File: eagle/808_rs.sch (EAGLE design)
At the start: 75 parts, among them IC1 TL072P, IC2 TL072P, Q1 2SK30, Q59 2N3904, Q60 2N3906, Q61 2N3904, Q62 2N3904, Q63 2N3904, SW8 808_LT_MSS42_SW_4PDT

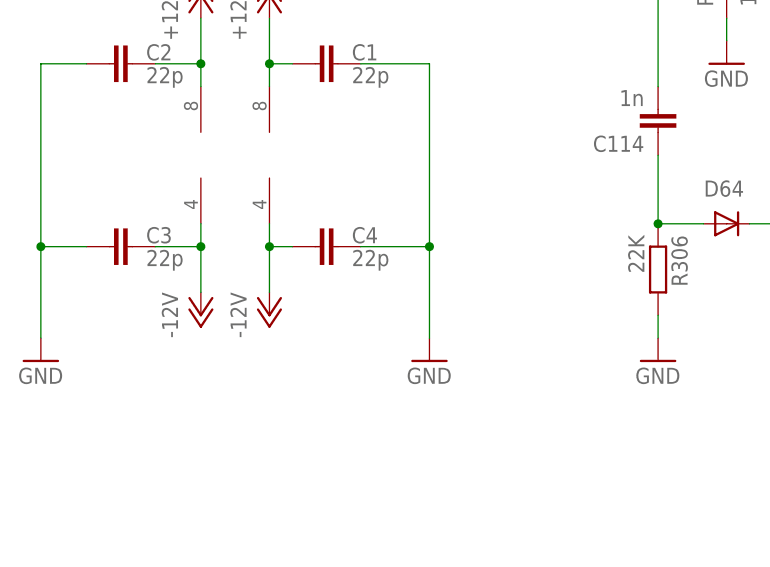
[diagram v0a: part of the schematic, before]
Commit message: 93pct auto
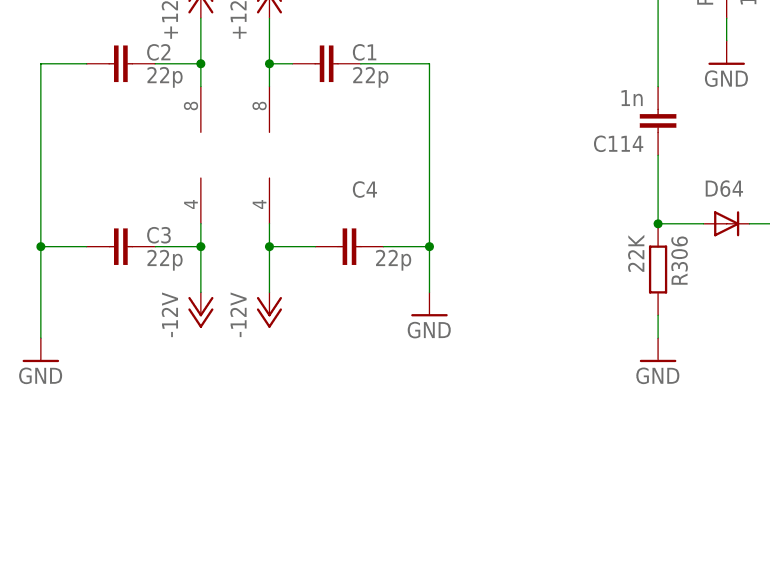
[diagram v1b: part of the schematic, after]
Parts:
- R305, R306, R310, R311, R316, R323, R324, R325, R326, R331: device TR808clone:R-EU_0207/5V -> TR808clone:R-EU_0207/7
- R313: device TR808clone:R-EU_0207/5V -> TR808clone:R-EU_0309/12
- R318: device TR808clone:R-EU_0207/5V -> TR808clone:R-EU_0207/2V
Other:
- moved on the sheet: C4

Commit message: 95pct auto
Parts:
- C113: device TR808clone:C-EU050-024X044 -> TR808clone:C-EU075-032X103
- C114: device TR808clone:C-EU3.5MM_PITCH -> TR808clone:C-EU050-030X075
- C121: device TR808clone:C-EU3.5MM_PITCH -> TR808clone:C-EU050-025X075
- C4: device TR808clone:C-EU025-025X050 -> TR808clone:C-EU050-024X044
- D61, D63, D64: value 1N4148DO35-7 -> 1N4148DO35-10; device TR808clone:1N4148DO35-7 -> TR808clone:1N4148DO35-10
- R303, R309, R330: device TR808clone:R-EU_0207/5V -> TR808clone:R-EU_0207/2V
- R316: device TR808clone:R-EU_0207/7 -> TR808clone:R-EU_0207/5V
- R321: device TR808clone:R-EU_0207/5V -> TR808clone:R-EU_0207/7
- R326: device TR808clone:R-EU_0207/7 -> TR808clone:R-EU_0309/10
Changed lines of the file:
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@@
 <part name="Q59" library="808_lt" deviceset="2N3904" device=""/>
 <part name="Q60" library="808_lt" deviceset="2N3906" device=""/>
-<part name="R303" library="TR808clone" deviceset="R-EU_" device="0207/5V" value="10K"/>
+<part name="R303" library="TR808clone" deviceset="R-EU_" device="0207/2V" value="10K"/>
 <part name="R297" library="TR808clone" deviceset="R-EU_" device="0207/5V" value="22K"/>
 <part name="R299" library="TR808clone" deviceset="R-EU_" device="0207/5V" value="4K7"/>
@@
 <part name="V200" library="supply1" deviceset="GND" device=""/>
 <part name="V201" library="supply1" deviceset="GND" device=""/>
-<part name="D61" library="TR808clone" deviceset="1N4148" device="DO35-7"/>
+<part name="D61" library="TR808clone" deviceset="1N4148" device="DO35-10" value="1N4148DO35-10"/>
 <part name="V202" library="supply1" deviceset="GND" device=""/>
 <part name="R107" library="TR808clone" deviceset="R-EU_" device="0207/5V" value="1K"/>
 <part name="V203" library="supply1" deviceset="GND" device=""/>
 <part name="R108" library="TR808clone" deviceset="R-EU_" device="0207/5V" value="10K"/>
-<part name="D63" library="TR808clone" deviceset="1N4148" device="DO35-7"/>
-<part name="C121" library="TR808clone" deviceset="C-EU" device="3.5MM_PITCH" value="4.7n"/>
+<part name="D63" library="TR808clone" deviceset="1N4148" device="DO35-10" value="1N4148DO35-10"/>
+<part name="C121" library="TR808clone" deviceset="C-EU" device="050-025X075" value="4.7n"/>
 <part name="C122" library="TR808clone" deviceset="C-EU" device="3.5MM_PITCH" value="4.7n"/>
 <part name="R325" library="TR808clone" deviceset="R-EU_" device="0207/7" value="330K"/>
@@
 <part name="V208" library="supply1" deviceset="GND" device=""/>
 <part name="R301" library="TR808clone" deviceset="R-EU_" device="0207/5V" value="47K"/>
-<part name="C114" library="TR808clone" deviceset="C-EU" device="3.5MM_PITCH" value="1n"/>
+<part name="C114" library="TR808clone" deviceset="C-EU" device="050-030X075" value="1n"/>
 <part name="R306" library="TR808clone" deviceset="R-EU_" device="0207/7" value="22K"/>
-<part name="D64" library="TR808clone" deviceset="1N4148" device="DO35-7"/>
+<part name="D64" library="TR808clone" deviceset="1N4148" device="DO35-10" value="1N4148DO35-10"/>
 <part name="R310" library="TR808clone" deviceset="R-EU_" device="0207/7" value="33K"/>
 <part name="R311" library="TR808clone" deviceset="R-EU_" device="0207/7" value="10K"/>
@@
 <part name="R313" library="TR808clone" deviceset="R-EU_" device="0309/12" value="390K"/>
 <part name="V212" library="supply1" deviceset="GND" device=""/>
-<part name="R309" library="TR808clone" deviceset="R-EU_" device="0207/5V" value="33K"/>
+<part name="R309" library="TR808clone" deviceset="R-EU_" device="0207/2V" value="33K"/>
 <part name="R319" library="TR808clone" deviceset="R-EU_" device="0207/5V" value="220K"/>
 <part name="C125" library="TR808clone" deviceset="C-EU" device="3.5MM_PITCH" value="10n"/>
-<part name="R326" library="TR808clone" deviceset="R-EU_" device="0207/7" value="10K"/>
+<part name="R326" library="TR808clone" deviceset="R-EU_" device="0309/10" value="10K"/>
 <part name="R331" library="TR808clone" deviceset="R-EU_" device="0207/7" value="47K"/>
 <part name="V213" library="supply1" deviceset="GND" device=""/>
 <part name="C153" library="TR808clone" deviceset="C-EU" device="025-025X050" value="22p"/>
-<part name="R330" library="TR808clone" deviceset="R-EU_" device="0207/5V" value="470K"/>
+<part name="R330" library="TR808clone" deviceset="R-EU_" device="0207/2V" value="470K"/>
 <part name="C126" library="TR808clone" deviceset="CPOL-EU" device="E2.5-5" value="33/6.3"/>
 <part name="C116" library="TR808clone" deviceset="C-EU" device="3.5MM_PITCH" value="4.7n"/>
@@
 <part name="R315" library="TR808clone" deviceset="R-EU_" device="0207/5V" value="5K6"/>
 <part name="V214" library="supply1" deviceset="GND" device=""/>
-<part name="R316" library="TR808clone" deviceset="R-EU_" device="0207/7" value="1M"/>
+<part name="R316" library="TR808clone" deviceset="R-EU_" device="0207/5V" value="1M"/>
 <part name="R318" library="TR808clone" deviceset="R-EU_" device="0207/2V" value="220K"/>
 <part name="R317" library="TR808clone" deviceset="R-EU_" device="0207/5V" value="10K"/>
 <part name="Q62" library="808_lt" deviceset="2N3904" device=""/>
 <part name="V215" library="supply1" deviceset="GND" device=""/>
-<part name="R321" library="TR808clone" deviceset="R-EU_" device="0207/5V" value="2M2"/>
+<part name="R321" library="TR808clone" deviceset="R-EU_" device="0207/7" value="2M2"/>
 <part name="C120" library="TR808clone" deviceset="CPOL-EU" device="E2.5-5" value="10/16"/>
 <part name="V217" library="supply1" deviceset="GND" device=""/>
@@
 <part name="Q61" library="808_lt" deviceset="2N3904" device=""/>
 <part name="C112" library="TR808clone" deviceset="C-EU" device="050-024X044" value="22n"/>
-<part name="C113" library="TR808clone" deviceset="C-EU" device="050-024X044" value="47n"/>
+<part name="C113" library="TR808clone" deviceset="C-EU" device="075-032X103" value="47n"/>
 <part name="R304" library="TR808clone" deviceset="R-EU_" device="0207/5V" value="47K"/>
 <part name="R305" library="TR808clone" deviceset="R-EU_" device="0207/7" value="1M"/>
@@
 <part name="C2" library="TR808clone" deviceset="C-EU" device="025-025X050" value="22p"/>
 <part name="C3" library="TR808clone" deviceset="C-EU" device="025-025X050" value="22p"/>
-<part name="C4" library="TR808clone" deviceset="C-EU" device="025-025X050" value="22p"/>
+<part name="C4" library="TR808clone" deviceset="C-EU" device="050-024X044" value="22p"/>
 <part name="TRIGGER" library="solpad" deviceset="LSP11" device=""/>
 <part name="SW8" library="808_lt" deviceset="808_LT_MSS42_SW_4PDT" device=""/>

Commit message: 94pct auto
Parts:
- C118: device TR808clone:C-EU3.5MM_PITCH -> TR808clone:C-EU050-024X044
- C122: device TR808clone:C-EU3.5MM_PITCH -> TR808clone:C-EU050-030X075
- R318: device TR808clone:R-EU_0207/2V -> TR808clone:R-EU_0207/5V
- R320, R322: device TR808clone:R-EU_0207/5V -> TR808clone:R-EU_0207/7
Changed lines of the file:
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@@
 <part name="D63" library="TR808clone" deviceset="1N4148" device="DO35-10" value="1N4148DO35-10"/>
 <part name="C121" library="TR808clone" deviceset="C-EU" device="050-025X075" value="4.7n"/>
-<part name="C122" library="TR808clone" deviceset="C-EU" device="3.5MM_PITCH" value="4.7n"/>
+<part name="C122" library="TR808clone" deviceset="C-EU" device="050-030X075" value="4.7n"/>
 <part name="R325" library="TR808clone" deviceset="R-EU_" device="0207/7" value="330K"/>
 <part name="Q63" library="808_lt" deviceset="2N3904" device=""/>
 <part name="R323" library="TR808clone" deviceset="R-EU_" device="0207/7" value="22K"/>
-<part name="R322" library="TR808clone" deviceset="R-EU_" device="0207/5V" value="10K"/>
+<part name="R322" library="TR808clone" deviceset="R-EU_" device="0207/7" value="10K"/>
 <part name="V204" library="supply1" deviceset="GND" device=""/>
 <part name="C111" library="TR808clone" deviceset="C-EU" device="3.5MM_PITCH" value="10n"/>
@@
 <part name="C119" library="TR808clone" deviceset="C-EU" device="3.5MM_PITCH" value="2.2n"/>
 <part name="C117" library="TR808clone" deviceset="C-EU" device="3.5MM_PITCH" value="2.2n"/>
-<part name="C118" library="TR808clone" deviceset="C-EU" device="3.5MM_PITCH" value="2.2n"/>
+<part name="C118" library="TR808clone" deviceset="C-EU" device="050-024X044" value="2.2n"/>
 <part name="R312" library="TR808clone" deviceset="R-EU_" device="0207/5V" value="1K"/>
 <part name="V211" library="supply1" deviceset="GND" device=""/>
@@
 <part name="V214" library="supply1" deviceset="GND" device=""/>
 <part name="R316" library="TR808clone" deviceset="R-EU_" device="0207/5V" value="1M"/>
-<part name="R318" library="TR808clone" deviceset="R-EU_" device="0207/2V" value="220K"/>
+<part name="R318" library="TR808clone" deviceset="R-EU_" device="0207/5V" value="220K"/>
 <part name="R317" library="TR808clone" deviceset="R-EU_" device="0207/5V" value="10K"/>
 <part name="Q62" library="808_lt" deviceset="2N3904" device=""/>
@@
 <part name="VR16" library="pot" deviceset="3RP/1610N" device="" value="100KA"/>
 <part name="R324" library="TR808clone" deviceset="R-EU_" device="0207/7" value="220K"/>
-<part name="R320" library="TR808clone" deviceset="R-EU_" device="0207/5V" value="22K"/>
+<part name="R320" library="TR808clone" deviceset="R-EU_" device="0207/7" value="22K"/>
 <part name="Q61" library="808_lt" deviceset="2N3904" device=""/>
 <part name="C112" library="TR808clone" deviceset="C-EU" device="050-024X044" value="22n"/>

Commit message: routed
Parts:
- C1: device TR808clone:C-EU025-025X050 -> TR808clone:C-EU050-024X044
- C112, C118: device TR808clone:C-EU050-024X044 -> TR808clone:C-EU050-025X075
- C113: device TR808clone:C-EU075-032X103 -> TR808clone:C-EU050-025X075
- C117, C119: device TR808clone:C-EU3.5MM_PITCH -> TR808clone:C-EU050-024X044
- C120: device TR808clone:CPOL-EUE2.5-5 -> TR808clone:CPOL-EUE2.5-6
- C125: device TR808clone:C-EU3.5MM_PITCH -> TR808clone:C-EU050-025X075
- R312, R314, R318: device TR808clone:R-EU_0207/5V -> TR808clone:R-EU_0207/7
- R331: device TR808clone:R-EU_0207/7 -> TR808clone:R-EU_0207/5V
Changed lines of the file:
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@@
 <part name="V210" library="supply1" deviceset="GND" device=""/>
 <part name="R308" library="TR808clone" deviceset="R-EU_" device="0207/5V" value="820K"/>
-<part name="C119" library="TR808clone" deviceset="C-EU" device="3.5MM_PITCH" value="2.2n"/>
-<part name="C117" library="TR808clone" deviceset="C-EU" device="3.5MM_PITCH" value="2.2n"/>
-<part name="C118" library="TR808clone" deviceset="C-EU" device="050-024X044" value="2.2n"/>
-<part name="R312" library="TR808clone" deviceset="R-EU_" device="0207/5V" value="1K"/>
+<part name="C119" library="TR808clone" deviceset="C-EU" device="050-024X044" value="2.2n"/>
+<part name="C117" library="TR808clone" deviceset="C-EU" device="050-024X044" value="2.2n"/>
+<part name="C118" library="TR808clone" deviceset="C-EU" device="050-025X075" value="2.2n"/>
+<part name="R312" library="TR808clone" deviceset="R-EU_" device="0207/7" value="1K"/>
 <part name="V211" library="supply1" deviceset="GND" device=""/>
-<part name="R314" library="TR808clone" deviceset="R-EU_" device="0207/5V" value="33K"/>
+<part name="R314" library="TR808clone" deviceset="R-EU_" device="0207/7" value="33K"/>
 <part name="R313" library="TR808clone" deviceset="R-EU_" device="0309/12" value="390K"/>
 <part name="V212" library="supply1" deviceset="GND" device=""/>
 <part name="R309" library="TR808clone" deviceset="R-EU_" device="0207/2V" value="33K"/>
 <part name="R319" library="TR808clone" deviceset="R-EU_" device="0207/5V" value="220K"/>
-<part name="C125" library="TR808clone" deviceset="C-EU" device="3.5MM_PITCH" value="10n"/>
+<part name="C125" library="TR808clone" deviceset="C-EU" device="050-025X075" value="10n"/>
 <part name="R326" library="TR808clone" deviceset="R-EU_" device="0309/10" value="10K"/>
-<part name="R331" library="TR808clone" deviceset="R-EU_" device="0207/7" value="47K"/>
+<part name="R331" library="TR808clone" deviceset="R-EU_" device="0207/5V" value="47K"/>
 <part name="V213" library="supply1" deviceset="GND" device=""/>
 <part name="C153" library="TR808clone" deviceset="C-EU" device="025-025X050" value="22p"/>
@@
 <part name="V214" library="supply1" deviceset="GND" device=""/>
 <part name="R316" library="TR808clone" deviceset="R-EU_" device="0207/5V" value="1M"/>
-<part name="R318" library="TR808clone" deviceset="R-EU_" device="0207/5V" value="220K"/>
+<part name="R318" library="TR808clone" deviceset="R-EU_" device="0207/7" value="220K"/>
 <part name="R317" library="TR808clone" deviceset="R-EU_" device="0207/5V" value="10K"/>
 <part name="Q62" library="808_lt" deviceset="2N3904" device=""/>
 <part name="V215" library="supply1" deviceset="GND" device=""/>
 <part name="R321" library="TR808clone" deviceset="R-EU_" device="0207/7" value="2M2"/>
-<part name="C120" library="TR808clone" deviceset="CPOL-EU" device="E2.5-5" value="10/16"/>
+<part name="C120" library="TR808clone" deviceset="CPOL-EU" device="E2.5-6" value="10/16"/>
 <part name="V217" library="supply1" deviceset="GND" device=""/>
 <part name="R300" library="TR808clone" deviceset="R-EU_" device="0207/5V" value="22K"/>
@@
 <part name="R320" library="TR808clone" deviceset="R-EU_" device="0207/7" value="22K"/>
 <part name="Q61" library="808_lt" deviceset="2N3904" device=""/>
-<part name="C112" library="TR808clone" deviceset="C-EU" device="050-024X044" value="22n"/>
-<part name="C113" library="TR808clone" deviceset="C-EU" device="075-032X103" value="47n"/>
+<part name="C112" library="TR808clone" deviceset="C-EU" device="050-025X075" value="22n"/>
+<part name="C113" library="TR808clone" deviceset="C-EU" device="050-025X075" value="47n"/>
 <part name="R304" library="TR808clone" deviceset="R-EU_" device="0207/5V" value="47K"/>
 <part name="R305" library="TR808clone" deviceset="R-EU_" device="0207/7" value="1M"/>
@@
 <part name="V2" library="supply1" deviceset="GND" device=""/>
 <part name="V3" library="supply1" deviceset="GND" device=""/>
-<part name="C1" library="TR808clone" deviceset="C-EU" device="025-025X050" value="22p"/>
+<part name="C1" library="TR808clone" deviceset="C-EU" device="050-024X044" value="22p"/>
 <part name="C2" library="TR808clone" deviceset="C-EU" device="025-025X050" value="22p"/>
 <part name="C3" library="TR808clone" deviceset="C-EU" device="025-025X050" value="22p"/>
